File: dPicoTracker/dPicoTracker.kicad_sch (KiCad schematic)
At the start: 9 parts, among them P1 USB_C_Plug_USB2.0, U1 RP2040, U2 LT1963AxST-3.3

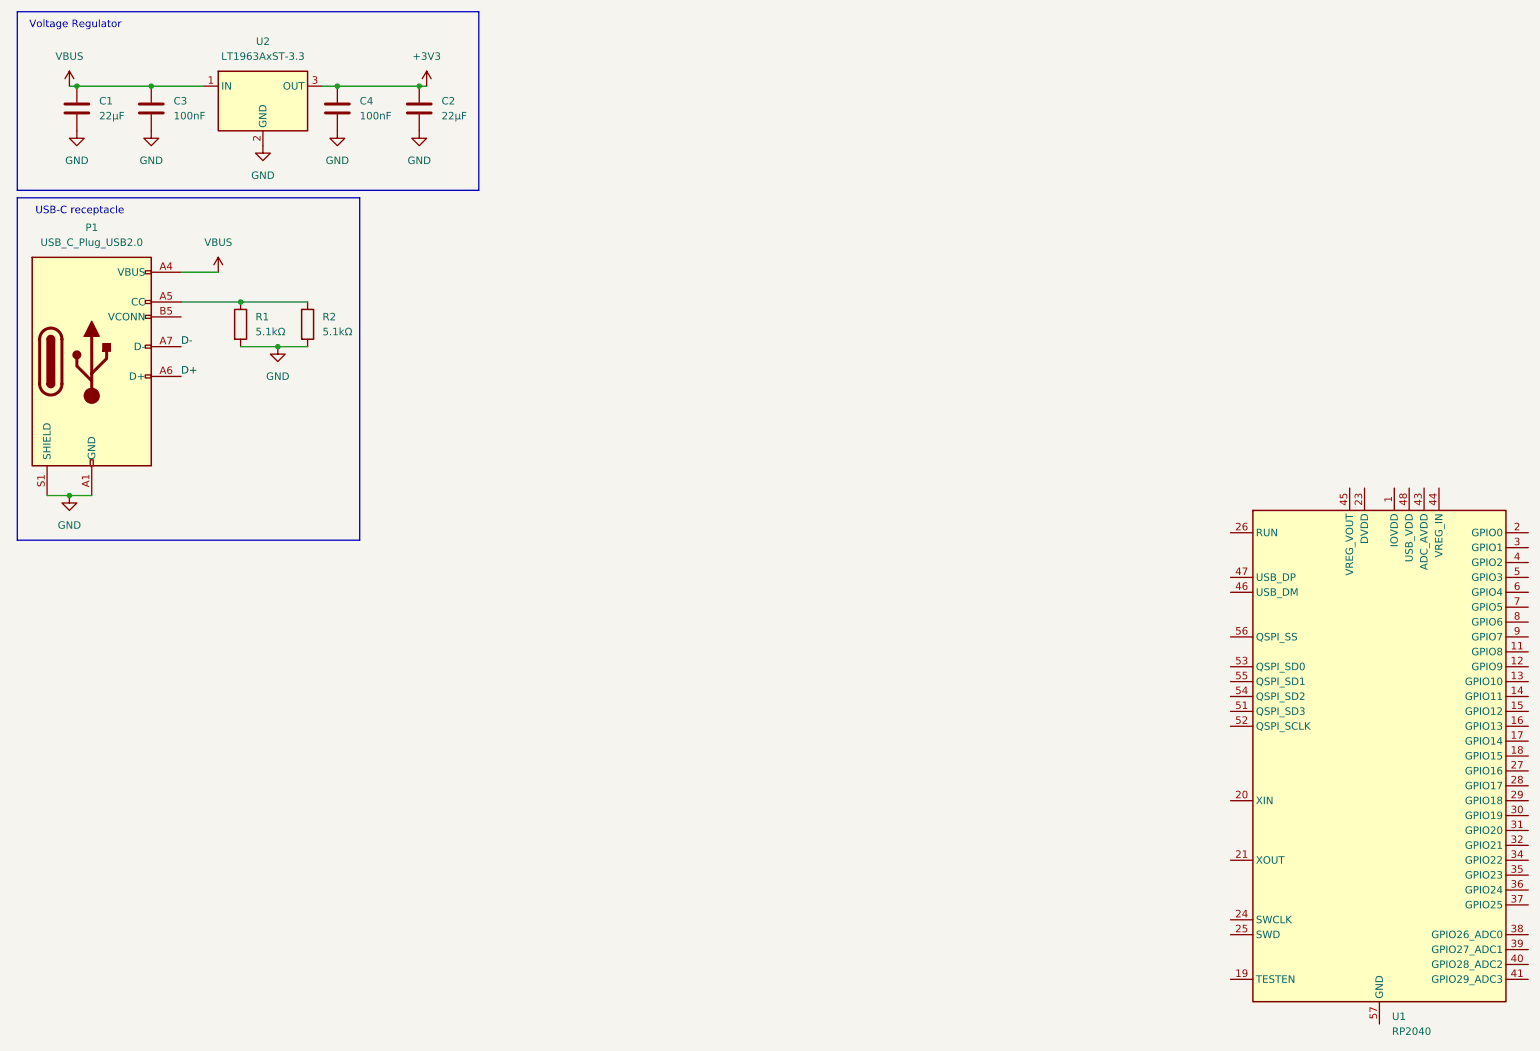
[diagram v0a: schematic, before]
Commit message: I think halfway there
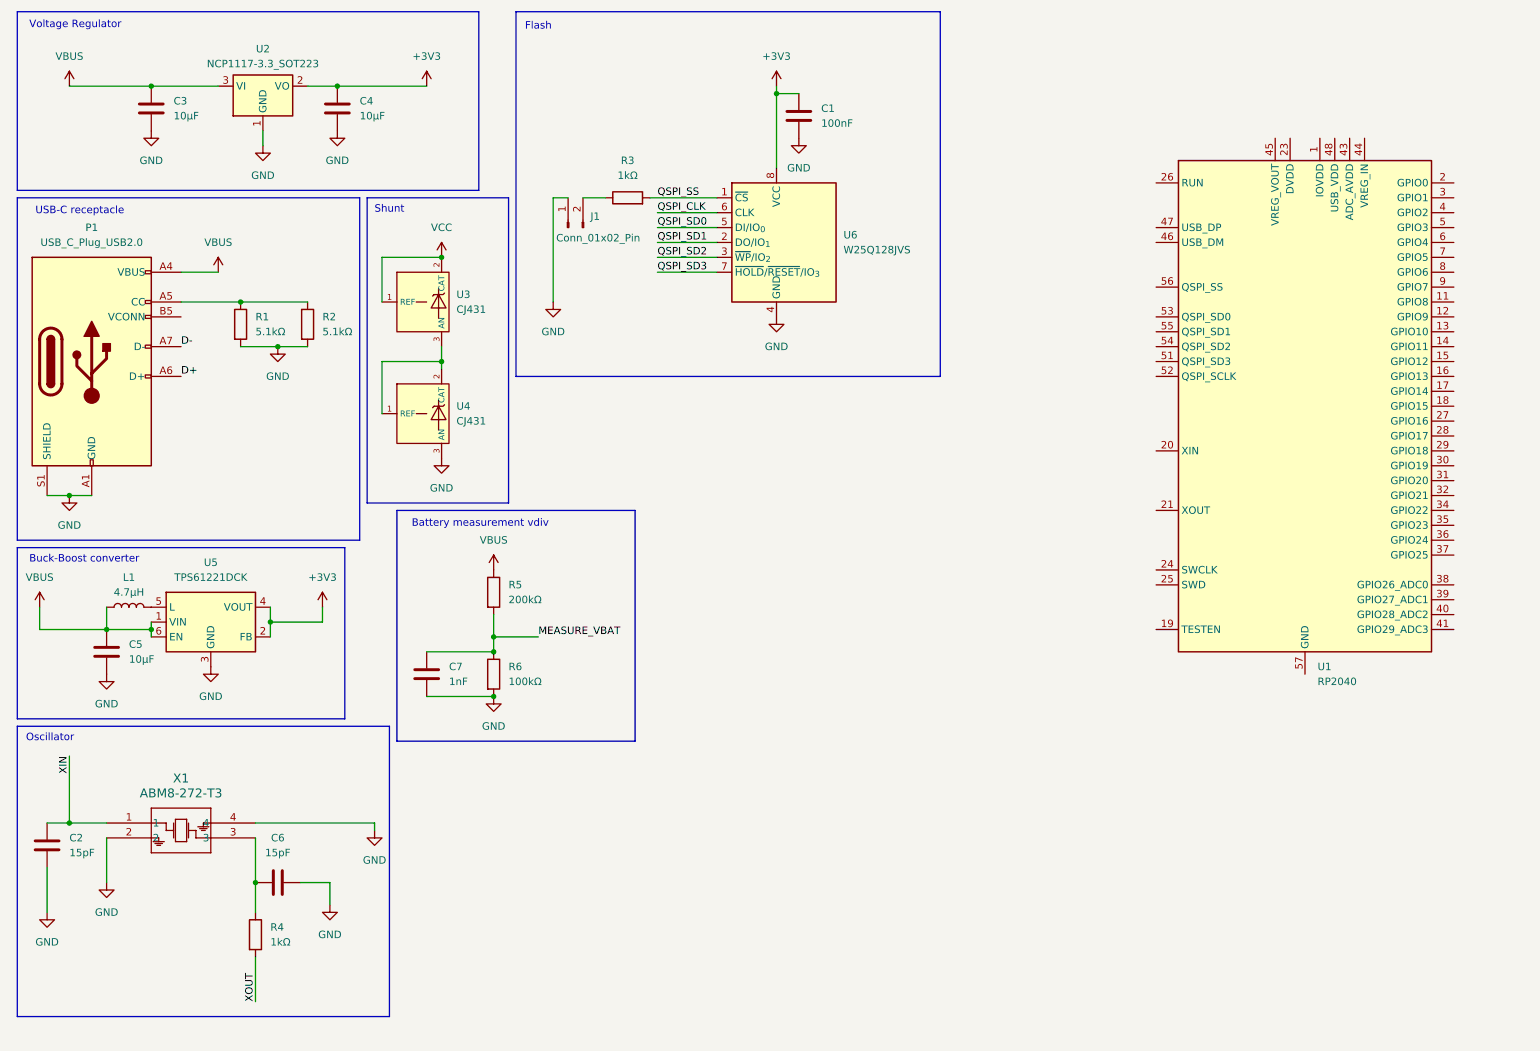
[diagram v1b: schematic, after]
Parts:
- removed U2: LT1963AxST-3.3, Package_TO_SOT_SMD:SOT-223-3_TabPin2, symbol Regulator_Linear:LT1963AxST-3.3
- added C5: 10µF, symbol Device:C
- added C6: 15pF, symbol Device:C
- added C7: 1nF, symbol Device:C
- added J1: Conn_01x02_Pin, Connector_PinHeader_2.00mm:PinHeader_1x02_P2.00mm_Vertical, symbol Connector:Conn_01x02_Pin
- added L1: 4.7µH, Inductor_SMD:L_1210_3225Metric, symbol Device:L
- added R3, R4: 1kΩ, symbol Device:R
- added R5: 200kΩ, symbol Device:R
- added R6: 100kΩ, symbol Device:R
- added U2: NCP1117-3.3_SOT223, Package_TO_SOT_SMD:SOT-223-3_TabPin2, symbol Regulator_Linear:NCP1117-3.3_SOT223
- added U3, U4: CJ431, PCM_JLCPCB:SOT-23-3_L2.9-W1.6-P1.90-LS2.8-BR, symbol PCM_JLCPCB-Power:Ref, 2-36V, 100mA, CJ431
- added U5: TPS61221DCK, Package_TO_SOT_SMD:SOT-23-5, symbol Regulator_Switching:TPS61221DCK
- added U6: W25Q128JVS, Package_SO:SOIC-8_5.3x5.3mm_P1.27mm, symbol Memory_Flash:W25Q128JVS
- added X1: ABM8-272-T3, ABM8-272-T3_ABR, symbol 2025-03-29_06-13-32:ABM8-272-T3
- C1: value 22µF -> 100nF
- C2: value 22µF -> 15pF
- C3, C4: value 100nF -> 10µF
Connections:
- net +3V3: now also C1.1, U2.2 (VO), U5.2 (FB), U5.4 (VOUT), U6.8 (VCC); no longer C2.1
- net GND: now also C2.1, C5.2, C6.2, C7.1, J1.1 (Pin_1), R6.2, U2.1 (GND), U4.3 (AN), U5.3 (GND), U6.4 (GND), X1.2, X1.4; no longer C2.2
- net VBUS: now also C5.1, L1.1, R5.1, U2.3 (VI), U5.1 (VIN), U5.6 (EN); no longer C1.1
- new net: L1.2, U5.5 (L)
- new net: J1.2 (Pin_2), R3.1
- new net: U3.3 (AN), U4.1 (REF), U4.2 (CAT)
- new net: C6.1, R4.1, X1.3
- new net MEASURE_VBAT: C7.2, R5.2, R6.1
- new net QSPI_CLK: U6.6 (CLK)
- new net QSPI_SD0: U6.5 (DI/IO_{0})
- new net QSPI_SD1: U6.2 (DO/IO_{1})
- new net QSPI_SD2: U6.3 (~{WP}/IO_{2})
- new net QSPI_SD3: U6.7 (~{HOLD}/~{RESET}/IO_{3})
- new net QSPI_SS: R3.2, U6.1 (~{CS})
- new net VCC: U3.1 (REF), U3.2 (CAT)
- new net XIN: C2.2, X1.1
- new net XOUT: R4.2
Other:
- note added: "Battery measurement vdiv"
- note added: "Buck-Boost converter"
- note added: "Flash"
- note added: "Oscillator"
- note added: "Shunt"
- moved on the sheet: U1
